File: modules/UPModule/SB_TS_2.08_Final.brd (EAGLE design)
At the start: 42.3 x 27.4 mm, 68 parts, among them IC1 MC34063AD, IC2 MCP1702-33, IC3 LPC922FDH, Q1 BC856, Q2 BCP52, Q4 ASFL, T1 BC848, T2 BC848

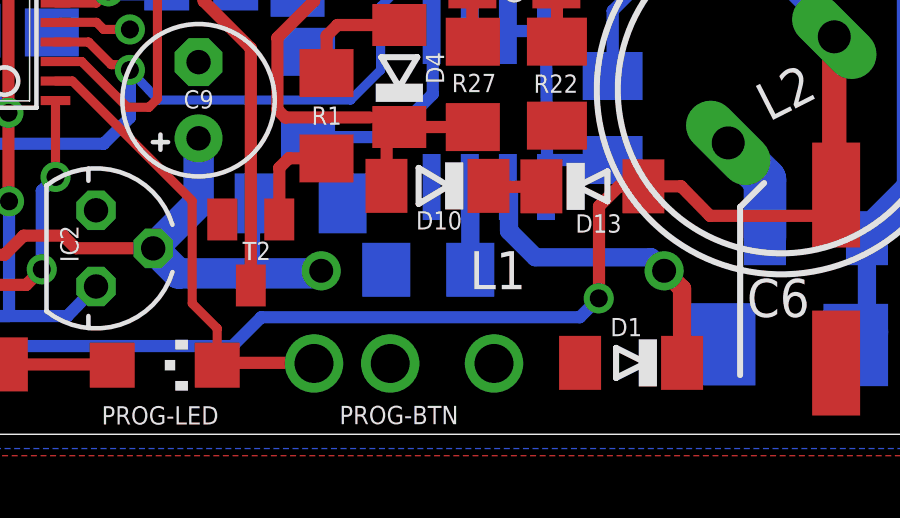
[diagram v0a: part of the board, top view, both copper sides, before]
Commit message: first upload TS-ARM3.05
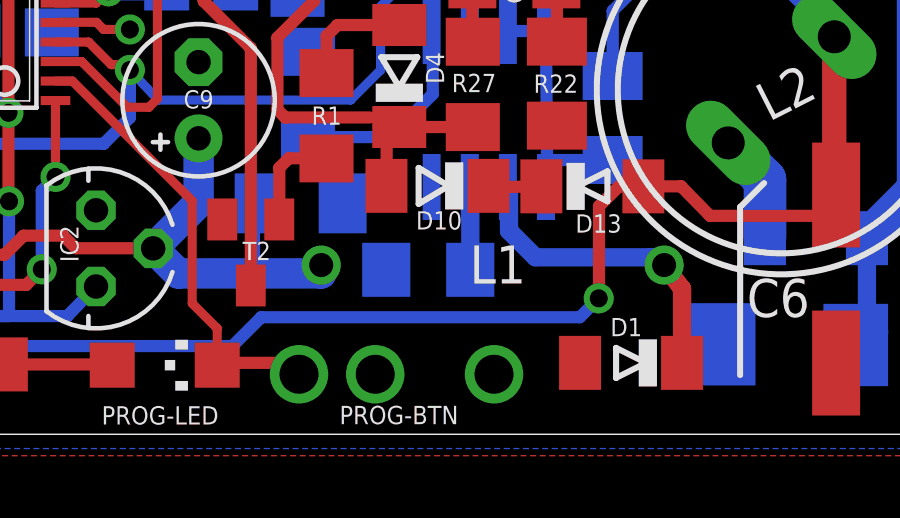
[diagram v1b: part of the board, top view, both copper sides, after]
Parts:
- moved L1 0.19 mm to (27.0, 5.64)
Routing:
- net PROG: track 15.8 -> 15.6 mm, vias 0 -> 1
